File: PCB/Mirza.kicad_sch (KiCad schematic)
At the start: 99 parts, among them J1 In, J2 Out, J3 Power, Q1 PMP5201Y, Q13 2SC3324, Q14 2SA1312, Q15 2SA1312, Q16 2SA1312, Q17 2SC3324, Q18 2SC3324, Q2 PMP4201Y, Q21 2SA1312, Q22 2SC3324, Q23 2SC3324, Q24 2SA1312, Q25 D45H11, Q26 D44H11, Q3 2SA1312, Q4 2SC3324, Q5 2SC3324, Q6 2SC3324, Q7 2SA1312, Q8 2SA1312, U1 OPA604

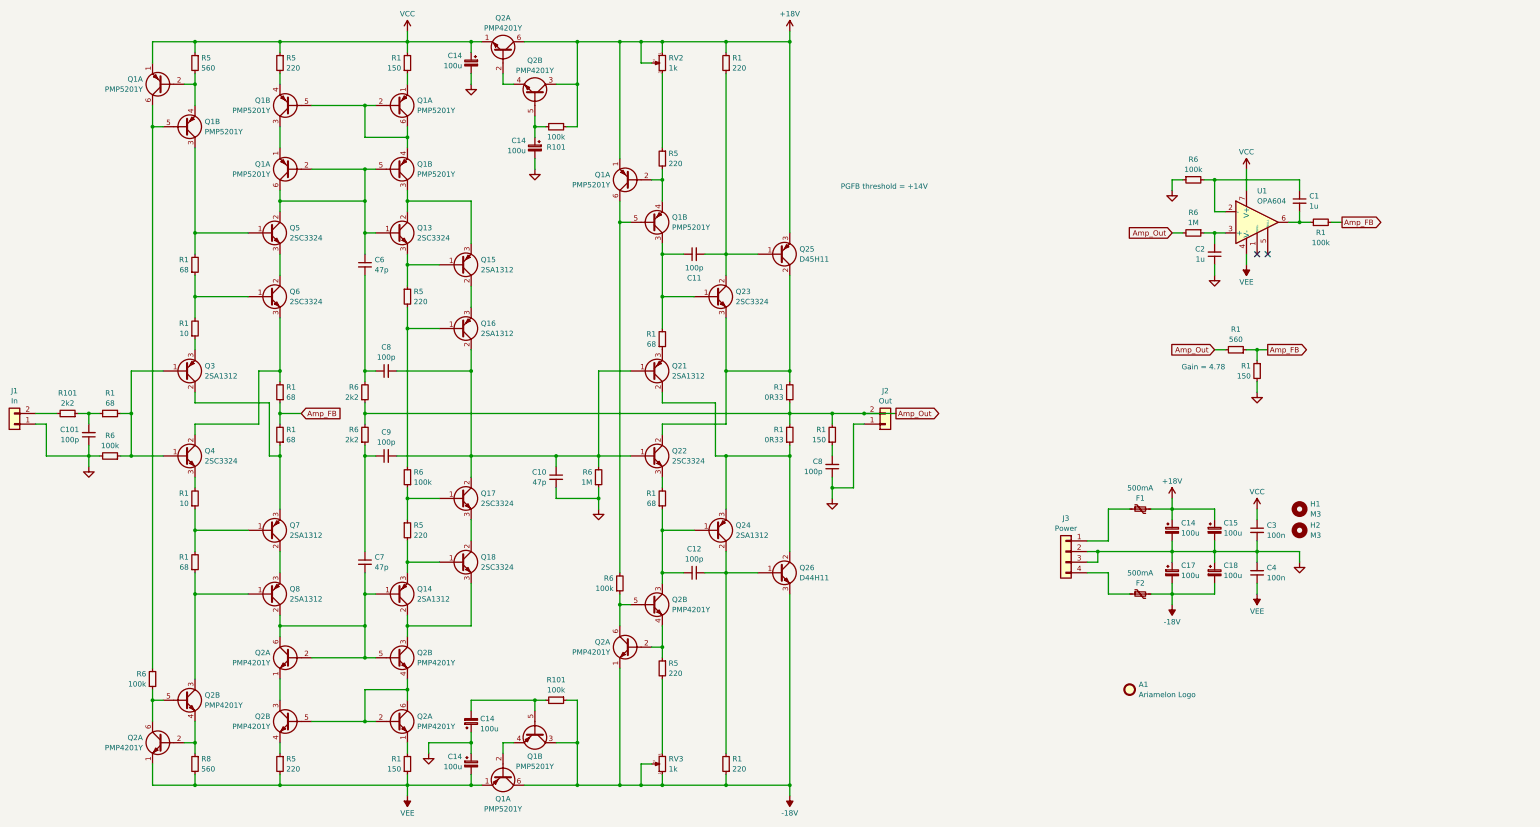
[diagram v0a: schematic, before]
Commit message: Initial public upload
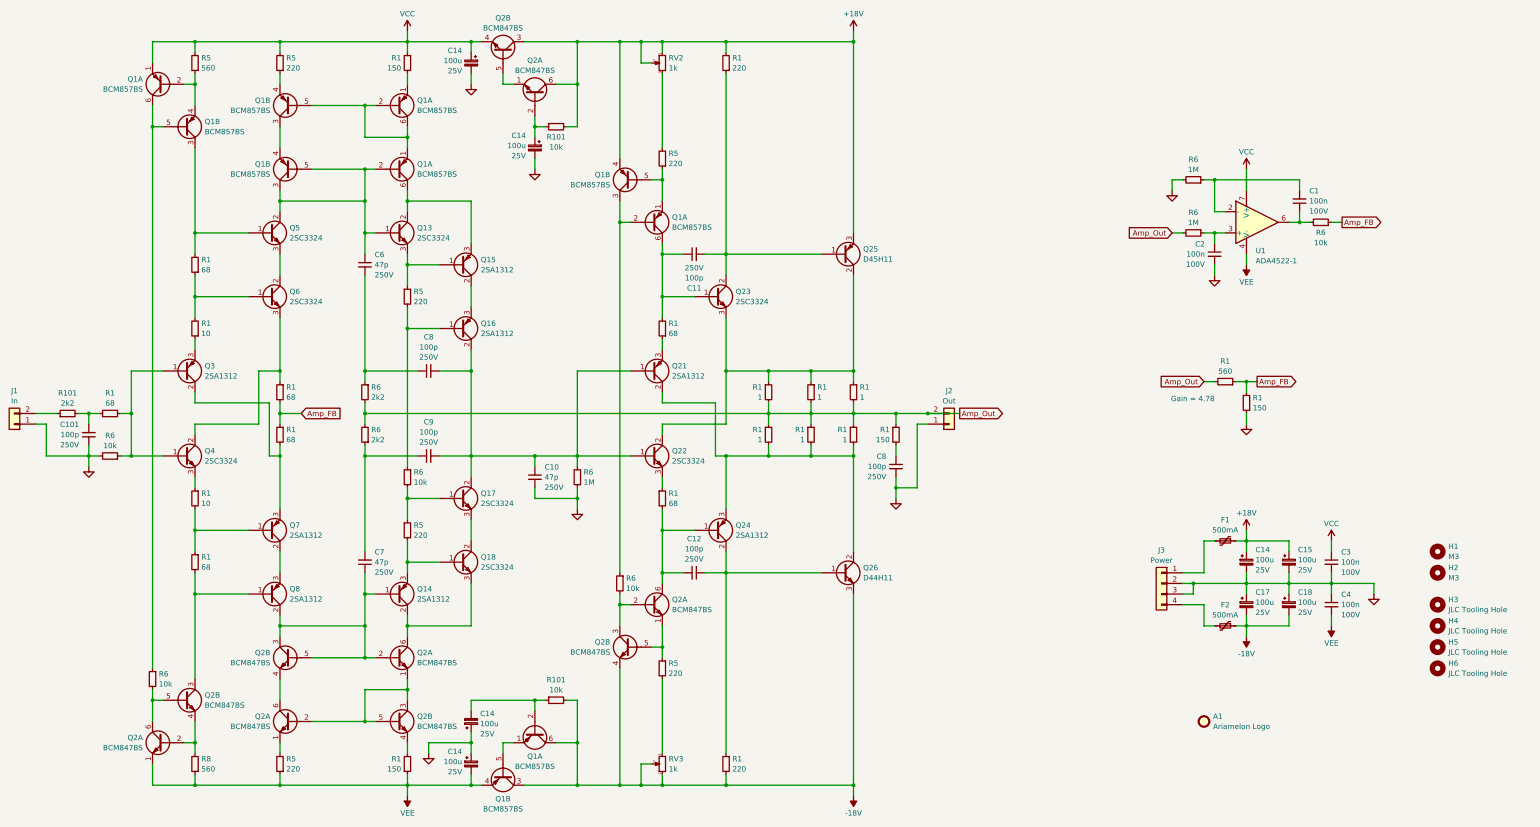
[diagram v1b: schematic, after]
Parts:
- removed R1, R6: 100k, Resistor_SMD:R_MiniMELF_MMA-0204, symbol Device:R_Small
- added H3, H4, H5, H6: JLC Tooling Hole, Ariamelon-HolePad:MountingHole_JLC-Tooling, symbol Mechanical:MountingHole
- added R1 (x4): 1, Resistor_SMD:R_MiniMELF_MMA-0204, symbol Device:R_Small
- added R6: 10k, Resistor_SMD:R_MiniMELF_MMA-0204, symbol Device:R_Small
- added R6: 1M, Resistor_SMD:R_MiniMELF_MMA-0204, symbol Device:R_Small
- C1, C2: value 1u -> 100n; LCSC (none) -> C85866; Manufacturer No. GRT21BR71H105KE01K -> GCM21BR72A104KA37L; Voltage (none) -> 100V
- C10, C6, C7: LCSC (none) -> C440149; Manufacturer No. 08052U470FAT2A -> GCM21A5C2E470JX01D; Voltage (none) -> 250V
- C101, C11, C12, C8, C9: LCSC (none) -> C437488; Manufacturer No. 08052U101FAT2A -> GCM21A7U2E101JX01D; Voltage (none) -> 250V
- C14, C15, C17, C18: footprint Capacitor_THT:CP_Radial_D6.3mm_P2.50mm -> Ariamelon-Device:CP_Radial_D6.3mm_P2.50mm; LCSC (none) -> C264049; Manufacturer No. EEU-FR1E151 -> EEUFR1E101; Voltage (none) -> 25V
- C3, C4: LCSC (none) -> C85866; Manufacturer No. GRT21BR71H104KE01L -> GCM21BR72A104KA37L; Voltage (none) -> 100V
- F1, F2: LCSC (none) -> C492011; Manufacturer No. 1206L050/24WR -> SMD1206P050TF/24
- H1, H2: footprint MountingHole:MountingHole_3.2mm_M3_Pad -> Ariamelon-HolePad:MountingHole_3.2mm_M3_Pad
- J1: now left out of the parts list
- Q1: value PMP5201Y -> BCM857BS; LCSC (none) -> C105887; Manufacturer No. PMP5201Y -> BCM857BS,115
- Q2: value PMP4201Y -> BCM847BS; LCSC (none) -> C396099; Manufacturer No. PMP4201Y -> BCM847BS,115
- Q2: value PMP4201Y -> BCM847BS; footprint Package_TO_SOT_SMD:SOT-363_SC-70-6 -> Ariamelon-Package:SOT-363_SC-70-6; LCSC (none) -> C396099; Manufacturer No. PMP4201Y -> BCM847BS,115
- Q25: Manufacturer No. (none) -> D45H11G
- Q26: Manufacturer No. (none) -> D44H11G
- R1: LCSC (none) -> C2074322; Manufacturer No. (none) -> MMA02040C1009FB300
- R1: LCSC (none) -> C2086951; Manufacturer No. (none) -> MMA02040C6809FB300
- R1, R5, R8: LCSC (none) -> C1884632; Manufacturer No. (none) -> MMA02040C5600FB300
- R1, R5: LCSC (none) -> C2074282; Manufacturer No. (none) -> MMA02040C2200FB300
- R1: LCSC (none) -> C2074241; Manufacturer No. (none) -> MMA02040C1500FB300
- R1: value 0R33 -> 1; footprint Resistor_SMD:R_MELF_MMB-0207 -> Resistor_SMD:R_MiniMELF_MMA-0204; LCSC (none) -> C2074959; Manufacturer No. (none) -> MMA02040C1008FB300
- R101, R6: LCSC (none) -> C1884620; Manufacturer No. (none) -> MMA02040C2201FB300
- R101, R6: value 100k -> 10k; LCSC (none) -> C2084764; Manufacturer No. (none) -> MMA02040C1002FB300
- R6: LCSC (none) -> C4339242; Manufacturer No. (none) -> MMA02040C1004FB300
- RV2, RV3: LCSC (none) -> C780233; Manufacturer No. (none) -> 3266W-1-102LF
- U1: value OPA604 -> ADA4522-1; LCSC (none) -> C160794; Manufacturer No. (none) -> ADA4522-1ARZ-R7
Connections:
- net +18V: now also F1.1, Q1.4 (E2), R101.2; no longer F1.2, Q1.1 (E1), R101.1
- net -18V: now also F2.1, Q2.4 (E2), R1.2, R101.2; no longer F2.2, Q2.1 (E1), R1.1, R101.1
- net Amp_FB: now also R1.1, R1.2, R1.2, R6.1; no longer R1.1, R1.1, R1.2
- net Amp_Out: now also R1.1, R1.1, R1.2, R6.2, R1.1, R1.1, R1.2, R1.2; no longer R1.1, R1.2, R1.2, R6.1
- net GND: now also C2.2, C4.1, C8.2, R1.1, R6.2; no longer C2.1, C4.2, C8.1, R1.2
- net VCC: now also Q2.4 (E2), R1.1, R5.2, R5.2; no longer Q2.1 (E1), R1.2, R5.1, R5.1
- net VEE: now also C4.2, Q1.4 (E2), R5.1, R8.1; no longer C4.1, Q1.1 (E1), R5.2, R8.2
- net at J3.1 (Pin_1): now also F1.2; no longer F1.1
- net at U1.6: now also C1.1, R6.2; no longer C1.2
- net at Q16.1 (B), R5.2: now also R6.1; no longer R6.2
- net at C11.1, Q23.1 (B), R1.2: now also Q1.6 (C1); no longer Q1.3 (C2)
- net at C101.2, R1.1: now also R101.2; no longer R101.1
- net at J1.2 (Pin_2): now also R101.1; no longer R101.2
- net at C9.1, R6.1: now also C7.2; no longer C7.1
- net at Q2.2 (B1): now also C14.1, R101.1; no longer Q2.4 (E2)
- net at C12.1, Q24.2 (C), Q26.1 (B): now also R1.1; no longer R1.2
- net at Q21.2 (C), Q24.3 (E), Q26.2 (C): now also R1.2, R1.2, R1.2; no longer R1.1
- net at Q17.1 (B), R5.1: now also R6.2; no longer R6.1
- net at Q1.2 (B1), Q1.4 (E2): now also R5.1; no longer R5.2
- net at Q1.5 (B2), Q1.6 (C1): now also R6.1; no longer R6.2
- net at Q2.1 (E1), Q2.3 (C2): now also Q2.2 (B1), Q2.5 (B2)
- net at Q2.4 (E2): now also R1.2; no longer R5.1
- net at Q2.4 (E2), Q2.6 (C1): no longer Q2.2 (B1), Q2.5 (B2)
- net at C12.2, Q24.1 (B): now also Q2.6 (C1), R1.2; no longer Q2.3 (C2), R1.1
- net at Q14.2 (C), Q18.3 (E): now also Q2.6 (C1); no longer Q2.3 (C2)
- net at R5.1: now also Q1.1 (E1), Q1.5 (B2); no longer RV2.3
- net at Q1.2 (B1): now also C14.2, R101.1; no longer Q1.4 (E2)
- net at U1.2 (-): now also C1.2, R6.1; no longer C1.1
- net at Q13.2 (C), Q15.3 (E): now also Q1.6 (C1); no longer Q1.3 (C2)
- net at Q1.2 (B1), Q1.5 (B2), Q1.6 (C1): now also Q1.1 (E1); no longer Q1.4 (E2)
- net at C6.1, Q1.2 (B1), Q1.5 (B2)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: now also Q1.3 (C2); no longer Q1.6 (C1)
- net at Q22.2 (C), Q23.3 (E), Q25.2 (C): now also R1.1, R1.1, R1.1; no longer R1.2
- net at Q22.3 (E): now also R1.1; no longer R1.2
- net at Q3.2 (C), Q7.3 (E): now also R1.2; no longer R1.1
- net at J3.4 (Pin_4): now also F2.2; no longer F2.1
- net at Q2.1 (E1): now also R5.2; no longer R1.2
- net at Q2.2 (B1), Q2.4 (E2): now also R8.2; no longer R8.1
- net at Q14.1 (B), Q2.2 (B1), Q2.5 (B2)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: now also C7.1, Q2.3 (C2); no longer C7.2, Q2.6 (C1)
- net at Q4.2 (C), Q6.3 (E): now also R1.1; no longer R1.2
- net at R1.2: now also Q7.1 (B), R1.1; no longer Q4.3 (E)
- net at Q2.3 (C2), Q8.1 (B): now also R1.2; no longer R1.1
- net at Q1.1 (E1): now also R1.2; no longer R1.1
- net at C6.2, C8.1: now also R6.1; no longer R6.2
- net at Q1.3 (C2): now also Q1.4 (E2); no longer Q1.1 (E1)
- net at Q1.4 (E2): now also R5.1; no longer R5.2
- net at Q2.5 (B2), Q2.6 (C1): now also R6.2; no longer R6.1
- net at R6.1, U1.3 (+): now also C2.1; no longer C2.2
- new net: Q1.2 (B1), Q1.3 (C2), R6.1
- new net: Q2.1 (E1), Q2.5 (B2)
- new net: Q2.2 (B1), Q2.3 (C2), R6.2
- new net: Q2.1 (E1), Q2.5 (B2), R5.1
- new net: R5.2, RV2.3
- new net: Q1.1 (E1), Q1.5 (B2)
- new net: C8.1, R1.2
- new net: Q4.3 (E), R1.1
- no-connect marks 2 -> 0
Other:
- note removed: "PGFB threshold = +14V"
- company: (none) -> Created by Ariamelon (https://github.com/Ariamelon/Mirza/)
- title: (none) -> Mirza Current-Feedback Amplifier Module
- moved on the sheet: A1, C10, C14, C15, C17, C18, C3, C4, C8, C9, F1, F2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
